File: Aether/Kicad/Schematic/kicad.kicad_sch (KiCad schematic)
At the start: 19 parts, among them IC1 AS5600-ASOT, U1 ESP32-S3-WROOM-1, U2 LM2596S-3.3, U3 SHT31-DIS, U4 BMP388, U5 SX1276, U6 ADS1115IDGS

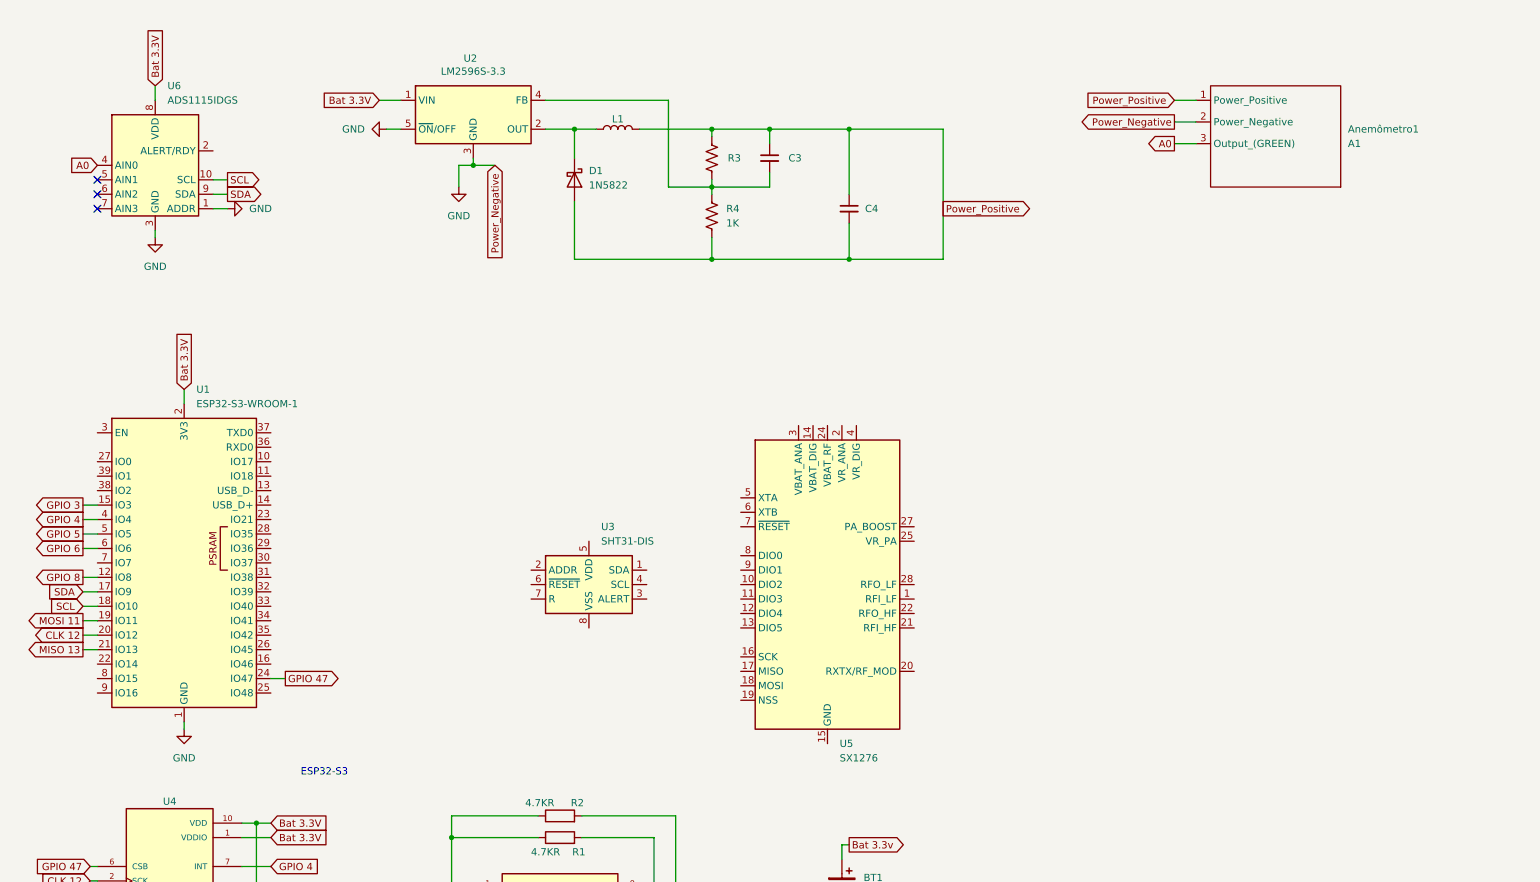
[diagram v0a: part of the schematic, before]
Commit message: Add files via upload
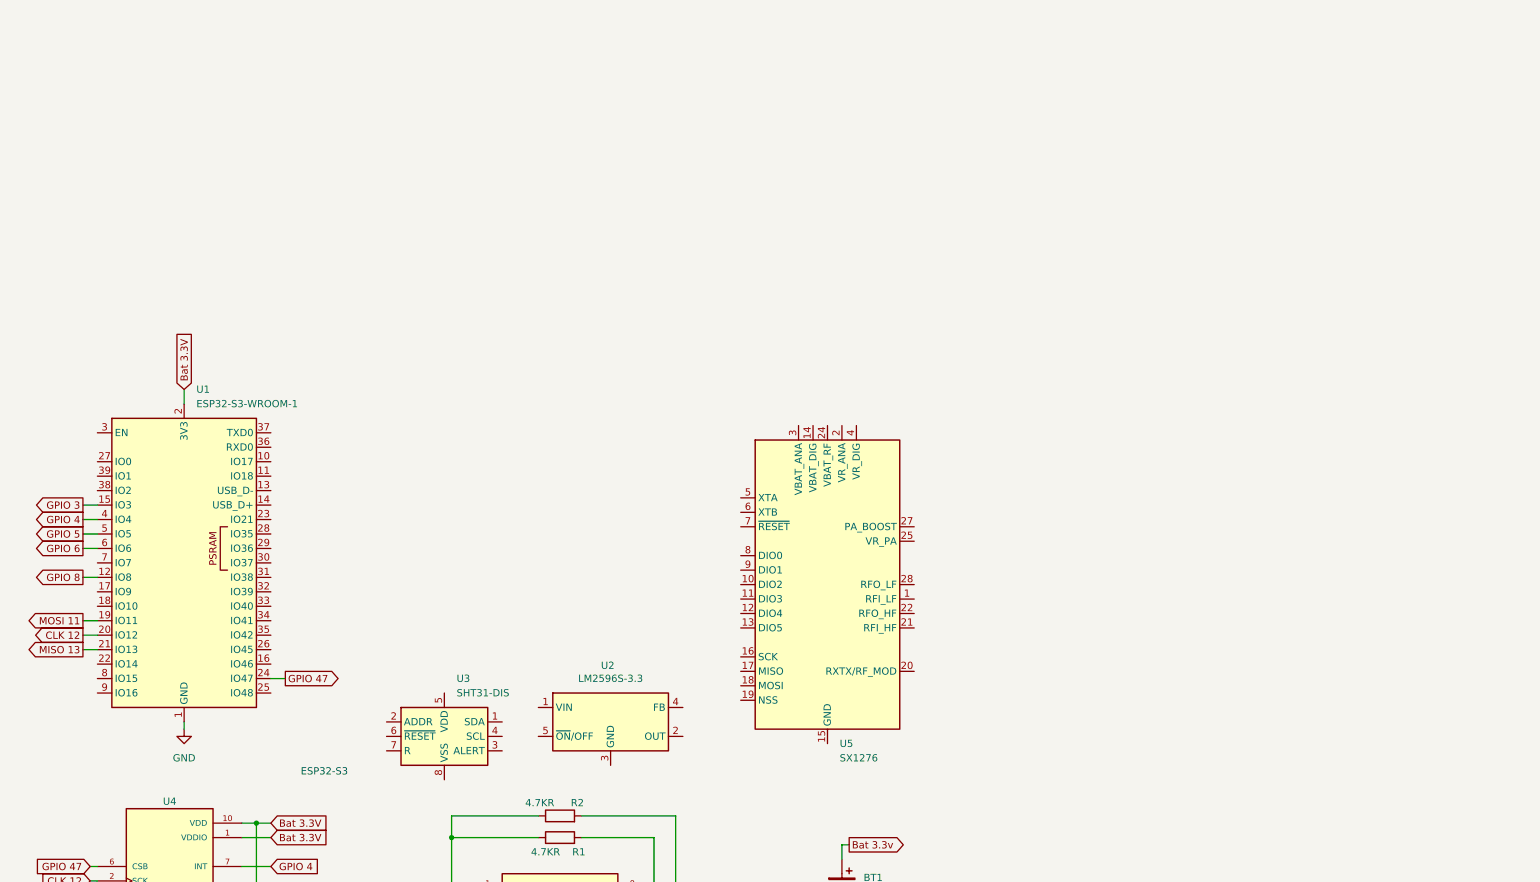
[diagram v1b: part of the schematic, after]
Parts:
- removed Anemômetro1: A1, symbol Anemômetro_analog:Anemômetro
- removed C3, C4: C_Small, symbol Device:C_Small
- removed D1: 1N5822, Diode_THT:D_DO-201AD_P15.24mm_Horizontal, symbol Diode:1N5822
- removed L1: L, symbol Device:L
- removed R3: R_US, symbol Device:R_US
- removed R4: 1K, symbol Device:R_US
- removed U6: ADS1115IDGS, Package_SO:TSSOP-10_3x3mm_P0.5mm, symbol Analog_ADC:ADS1115IDGS
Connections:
- net Bat 3.3V: no longer U2.1 (VIN)
- net GND: no longer U2.3 (GND), U2.5 (~{ON}/OFF)
- net SCL: no longer names the net of U1.18 (IO10)
- net SDA: no longer names the net of U1.17 (IO9)
- no-connect marks 4 -> 1
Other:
- moved on the sheet: U2, U3
